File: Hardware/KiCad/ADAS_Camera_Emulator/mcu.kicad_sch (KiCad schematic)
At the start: 9 parts, among them U1 STM32L476RGTx

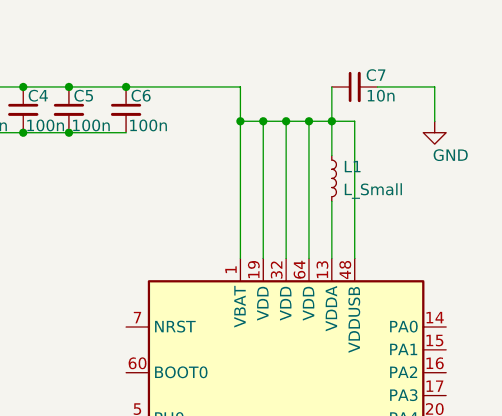
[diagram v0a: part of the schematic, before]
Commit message: just shematic stuff
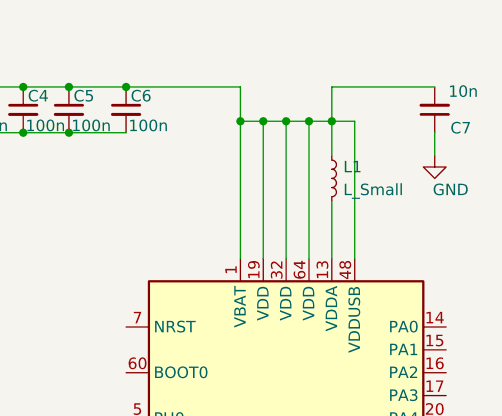
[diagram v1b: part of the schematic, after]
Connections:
- net +3.3V: now also C7.2; no longer C7.1
- net GND: now also C7.1; no longer C7.2
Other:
- moved on the sheet: C7
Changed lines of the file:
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@@
+	(wire
+		(pts
+			(xy 151.13 33.02) (xy 162.56 33.02)
+		)
+		(stroke
+			(width 0)
+			(type default)
+		)
+	)
 	(wire
 		(pts
@@
 	(wire
 		(pts
+			(xy 162.56 38.1) (xy 162.56 40.64)
+		)
+		(stroke
+			(width 0)
+			(type default)
+		)
+	)
+	(wire
+		(pts
 			(xy 146.05 52.07) (xy 146.05 36.83)
 		)
@@
 	(wire
 		(pts
-			(xy 162.56 36.83) (xy 162.56 33.02)
-		)
-		(stroke
-			(width 0)
-			(type default)
-		)
-	)
-	(wire
-		(pts
 			(xy 146.05 148.59) (xy 148.59 148.59)
 		)
@@
 		(pts
 			(xy 146.05 148.59) (xy 146.05 151.13)
-		)
-		(stroke
-			(width 0)
-			(type default)
-		)
-	)
-	(wire
-		(pts
-			(xy 162.56 33.02) (xy 156.21 33.02)
 		)
 		(stroke
@@
 	(symbol
 		(lib_id "Device:C_Small")
-		(at 153.67 33.02 90)
+		(at 162.56 35.56 180)
 		(unit 1)
 		(exclude_from_sim no)
@@
 		(dnp no)
 		(property "Reference" "C7"
-			(at 157.226 31.75 90)
+			(at 166.624 37.592 0)
 			(effects
 				(font
@@
 		)
 		(property "Value" "10n"
-			(at 158.242 34.036 90)
+			(at 167.386 33.528 0)
 			(effects
 				(font
@@
 		)
 		(property "Footprint" "Capacitor_SMD:C_0402_1005Metric"
-			(at 153.67 33.02 0)
+			(at 162.56 35.56 0)
 			(effects
 				(font
@@
 		)
 		(property "Datasheet" "~"
-			(at 153.67 33.02 0)
+			(at 162.56 35.56 0)
 			(effects
 				(font
@@
 		)
 		(property "Description" "Unpolarized capacitor, small symbol"
-			(at 153.67 33.02 0)
+			(at 162.56 35.56 0)
 			(effects
 				(font
@@
 	(symbol
 		(lib_id "power:GND")
-		(at 162.56 36.83 0)
+		(at 162.56 40.64 0)
 		(unit 1)
 		(exclude_from_sim no)
@@
 		(dnp no)
 		(property "Reference" "#PWR04"
-			(at 162.56 43.18 0)
+			(at 162.56 46.99 0)
 			(effects
 				(font
@@
 		)
 		(property "Value" "GND"
-			(at 164.338 40.64 0)
+			(at 164.338 44.45 0)
 			(effects
 				(font
@@
 		)
 		(property "Footprint" ""
-			(at 162.56 36.83 0)
+			(at 162.56 40.64 0)
 			(effects
 				(font
@@
 		)
 		(property "Datasheet" ""
-			(at 162.56 36.83 0)
+			(at 162.56 40.64 0)
 			(effects
 				(font
@@
 		)
 		(property "Description" "Power symbol creates a global label with name \"GND\" , ground"
-			(at 162.56 36.83 0)
-			(effects
-				(font
+			(at 162.56 40.64 0)
+			(effects
+				(font
